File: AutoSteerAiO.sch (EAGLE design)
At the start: 82 parts, among them J4 CONNECTOR 1x5 PINS, K4 CB1A-P-12V, U1 VX7805-1000

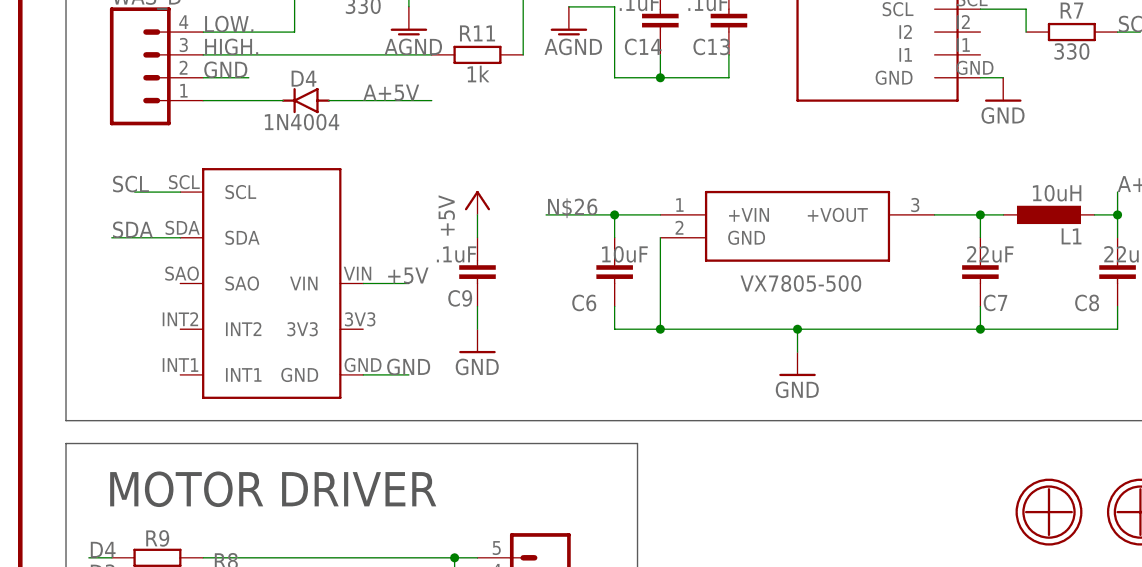
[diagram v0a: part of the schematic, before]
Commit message: Add files via upload
Adding jumper SAO
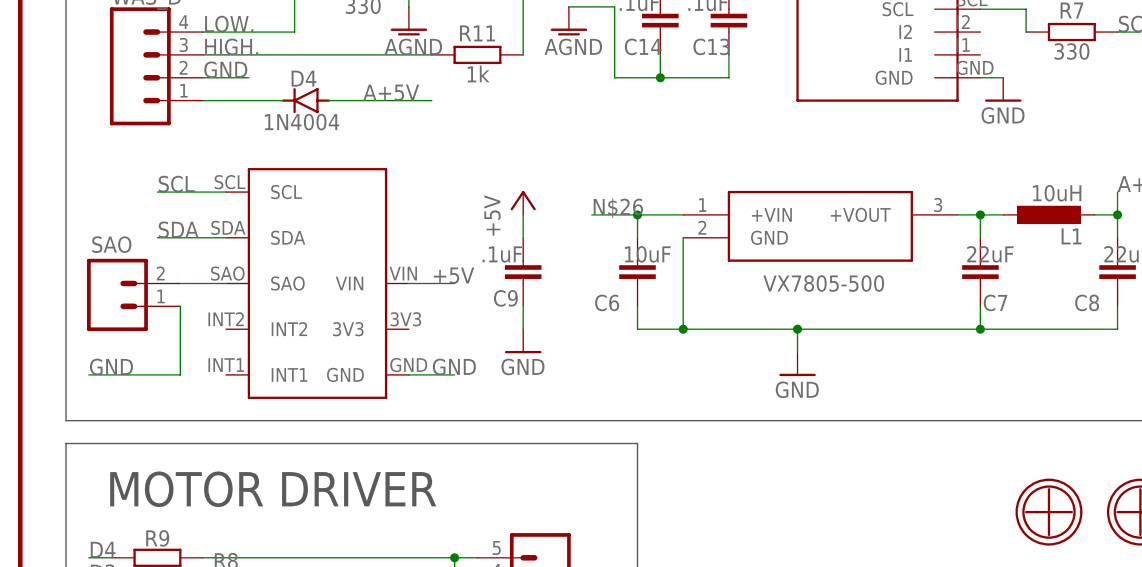
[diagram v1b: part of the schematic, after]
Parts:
- added SAO: CONNECTOR 1x2 PINS, SparkFun-Connectors:CONN_02
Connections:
- new net N$23: MMA8542.SAO, SAO.2
- net GND: now also SAO.1
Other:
- moved on the sheet: C6, C9
